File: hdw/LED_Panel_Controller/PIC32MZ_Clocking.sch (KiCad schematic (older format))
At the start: 17 parts, among them U1001 74LVC1G97, X1001 ASE-8.000MHz, X1002 ECS-327KE

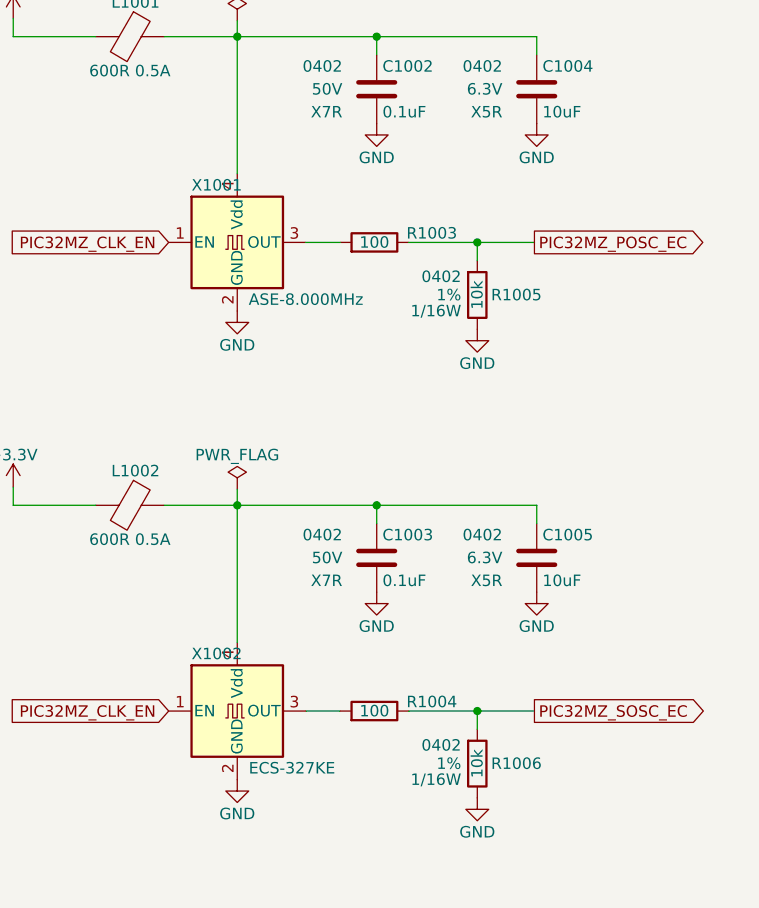
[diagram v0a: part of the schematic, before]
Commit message: reviewed schematic
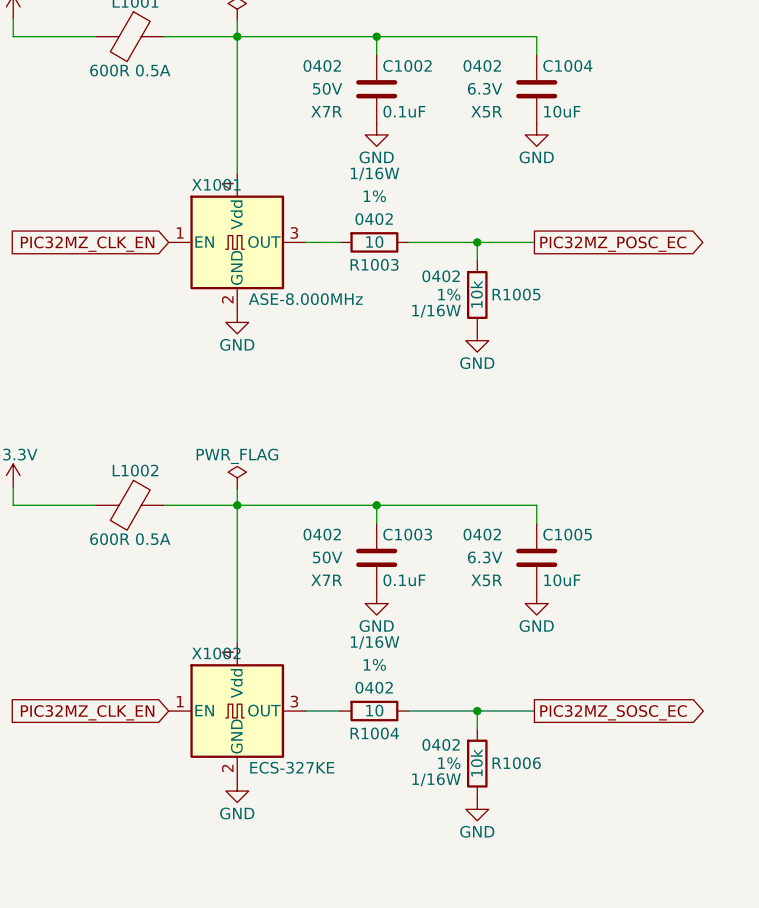
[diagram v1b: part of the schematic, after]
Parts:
- R1003, R1004: value 100 -> 10; Digi-Key PN RMCF0402FT100RCT-ND -> RMCF0402FT10R0CT-ND
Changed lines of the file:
@@
 Sheet 10 34
 Title "LED Panel Controller"
-Date "2021-03-24"
+Date "2021-03-31"
 Rev "A"
 Comp "Drew Maatman"
@@
 	6560 2700 6560 2780
 Connection ~ 6560 2700
-$Comp
-L Custom_Library:R_Custom R?
-U 1 1 5E024C29
-P 6110 2700
-AR Path="/5BAAE2B6/5E024C29" Ref="R?"  Part="1"
-AR Path="/5BB6CF6D/5E024C29" Ref="R?"  Part="1"
-AR Path="/5BBE424C/5E024C29" Ref="R?"  Part="1"
-AR Path="/5BAAE1DC/5E024C29" Ref="R?"  Part="1"
-AR Path="/5CAD2DA3/5E024C29" Ref="R?"  Part="1"
-AR Path="/5E01BCC3/5E024C29" Ref="R?"  Part="1"
-AR Path="/5E697952/5E024C29" Ref="R?"  Part="1"
-AR Path="/5EAE2F15/5E024C29" Ref="R?"  Part="1"
-AR Path="/5F5829C2/5E024C29" Ref="R1003"  Part="1"
-F 0 "R1003" V 6070 2560 50  0000 R CNN
-F 1 "100" V 6110 2700 50  0000 C CNN
-F 2 "Resistors_SMD:R_0402" H 6110 2700 50  0001 C CNN
-F 3 "" H 6110 2700 50  0001 C CNN
-F 4 "0402" V 6210 2700 50  0001 C CNN "display_footprint"
-F 5 "1%" V 6310 2700 50  0001 C CNN "Tolerance"
-F 6 "1/16W" V 6410 2700 50  0001 C CNN "Wattage"
-F 7 "RMCF0402FT100RCT-ND" H 6410 3100 60  0001 C CNN "Digi-Key PN"
-	1    6110 2700
-	0    -1   1    0
-$EndComp
 Wire Wire Line
 	5960 2700 5810 2700
@@
 	6560 4750 6560 4830
 Connection ~ 6560 4750
-$Comp
-L Custom_Library:R_Custom R?
-U 1 1 5F689623
-P 6110 4750
-AR Path="/5BAAE2B6/5F689623" Ref="R?"  Part="1"
-AR Path="/5BB6CF6D/5F689623" Ref="R?"  Part="1"
-AR Path="/5BBE424C/5F689623" Ref="R?"  Part="1"
-AR Path="/5BAAE1DC/5F689623" Ref="R?"  Part="1"
-AR Path="/5CAD2DA3/5F689623" Ref="R?"  Part="1"
-AR Path="/5E01BCC3/5F689623" Ref="R?"  Part="1"
-AR Path="/5E697952/5F689623" Ref="R?"  Part="1"
-AR Path="/5EAE2F15/5F689623" Ref="R?"  Part="1"
-AR Path="/5F5829C2/5F689623" Ref="R1004"  Part="1"
-F 0 "R1004" V 6070 4610 50  0000 R CNN
-F 1 "100" V 6110 4750 50  0000 C CNN
-F 2 "Resistors_SMD:R_0402" H 6110 4750 50  0001 C CNN
-F 3 "" H 6110 4750 50  0001 C CNN
-F 4 "0402" V 6210 4750 50  0001 C CNN "display_footprint"
-F 5 "1%" V 6310 4750 50  0001 C CNN "Tolerance"
-F 6 "1/16W" V 6410 4750 50  0001 C CNN "Wattage"
-F 7 "RMCF0402FT100RCT-ND" H 6410 5150 60  0001 C CNN "Digi-Key PN"
-	1    6110 4750
-	0    -1   1    0
-$EndComp
 Wire Wire Line
 	5960 4750 5810 4750
@@
 Text GLabel 5210 4750 0    50   Input ~ 0
 PIC32MZ_CLK_EN
+$Comp
+L Custom_Library:R_Custom R?
+U 1 1 606585C6
+P 6110 2700
+AR Path="/5F5829A6/606585C6" Ref="R?"  Part="1"
+AR Path="/5F5829C2/606585C6" Ref="R1003"  Part="1"
+F 0 "R1003" V 6010 2700 50  0000 C CNN
+F 1 "10" V 6110 2700 50  0000 C CNN
+F 2 "Resistors_SMD:R_0402" H 6110 2700 50  0001 C CNN
+F 3 "" H 6110 2700 50  0001 C CNN
+F 4 "0402" V 6210 2700 50  0000 C CNN "display_footprint"
+F 5 "1%" V 6310 2700 50  0000 C CNN "Tolerance"
+F 6 "1/16W" V 6410 2700 50  0000 C CNN "Wattage"
+F 7 "RMCF0402FT10R0CT-ND" H 6410 3100 60  0001 C CNN "Digi-Key PN"
+	1    6110 2700
+	0    -1   -1   0
+$EndComp
+$Comp
+L Custom_Library:R_Custom R?
+U 1 1 60658A20
+P 6110 4750
+AR Path="/5F5829A6/60658A20" Ref="R?"  Part="1"
+AR Path="/5F5829C2/60658A20" Ref="R1004"  Part="1"
+F 0 "R1004" V 6010 4750 50  0000 C CNN
+F 1 "10" V 6110 4750 50  0000 C CNN
+F 2 "Resistors_SMD:R_0402" H 6110 4750 50  0001 C CNN
+F 3 "" H 6110 4750 50  0001 C CNN
+F 4 "0402" V 6210 4750 50  0000 C CNN "display_footprint"
+F 5 "1%" V 6310 4750 50  0000 C CNN "Tolerance"
+F 6 "1/16W" V 6410 4750 50  0000 C CNN "Wattage"
+F 7 "RMCF0402FT10R0CT-ND" H 6410 5150 60  0001 C CNN "Digi-Key PN"
+	1    6110 4750
+	0    -1   -1   0
+$EndComp
 $EndSCHEMATC
